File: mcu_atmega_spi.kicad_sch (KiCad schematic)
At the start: 34 parts, among them J10 Conn_01x01, J5 AVR ICSP, J6 Conn_01x01, J7 Conn_01x01, J8 Conn_01x01, J9 Conn_01x01, SW1 SW_Push, SW2 SW_Push, SW3 SW_Push, U5 ATmega328P-A, U6 CP2102N-A02-GQFN28, Y2 Crystal_GND24

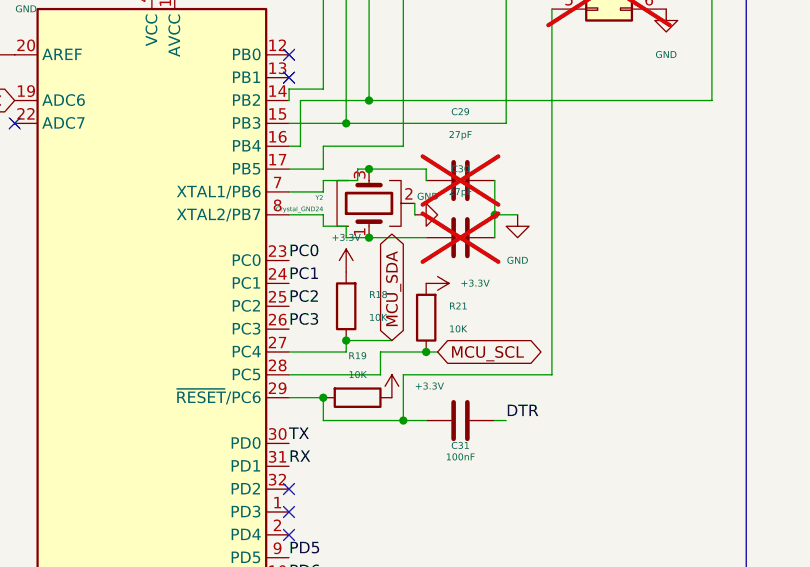
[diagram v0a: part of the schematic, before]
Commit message: .
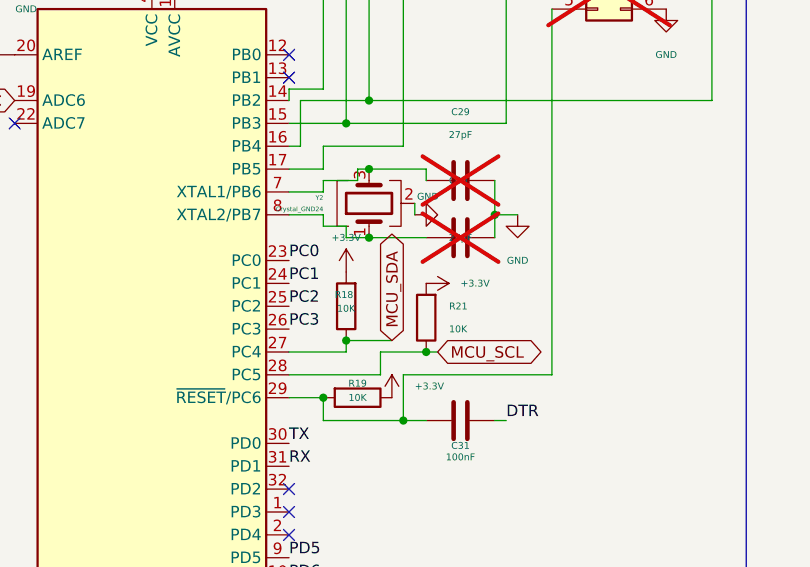
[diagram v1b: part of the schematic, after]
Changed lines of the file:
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@@
 		(in_pos_files yes)
 		(dnp yes)
-		(fields_autoplaced yes)
 		(property "Reference" "C30"
-			(at 130.81 85.09 90)
+			(at 130.556 86.36 90)
 			(show_name no)
 			(do_not_autoplace no)
@@
 		)
 		(property "Value" "27pF"
-			(at 130.81 87.63 90)
+			(at 130.81 92.71 90)
 			(show_name no)
 			(do_not_autoplace no)
@@
 		(dnp no)
 		(property "Reference" "R19"
-			(at 119.38 105.41 90)
+			(at 119.38 108.458 90)
 			(show_name no)
 			(do_not_autoplace no)
@@
 		)
 		(property "Value" "10K"
-			(at 119.38 107.95 90)
+			(at 119.38 110.49 90)
 			(show_name no)
 			(do_not_autoplace no)
@@
 		(in_pos_files yes)
 		(dnp no)
-		(fields_autoplaced yes)
 		(property "Reference" "R18"
-			(at 120.65 99.0599 0)
+			(at 116.84 99.06 0)
 			(show_name no)
 			(do_not_autoplace no)
@@
 		)
 		(property "Value" "10K"
-			(at 120.65 101.5999 0)
-			(show_name no)
-			(do_not_autoplace no)
+			(at 117.094 100.584 0)
+			(show_name no)
+			(do_not_autoplace no)
